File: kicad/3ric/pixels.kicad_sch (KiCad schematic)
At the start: 13 parts

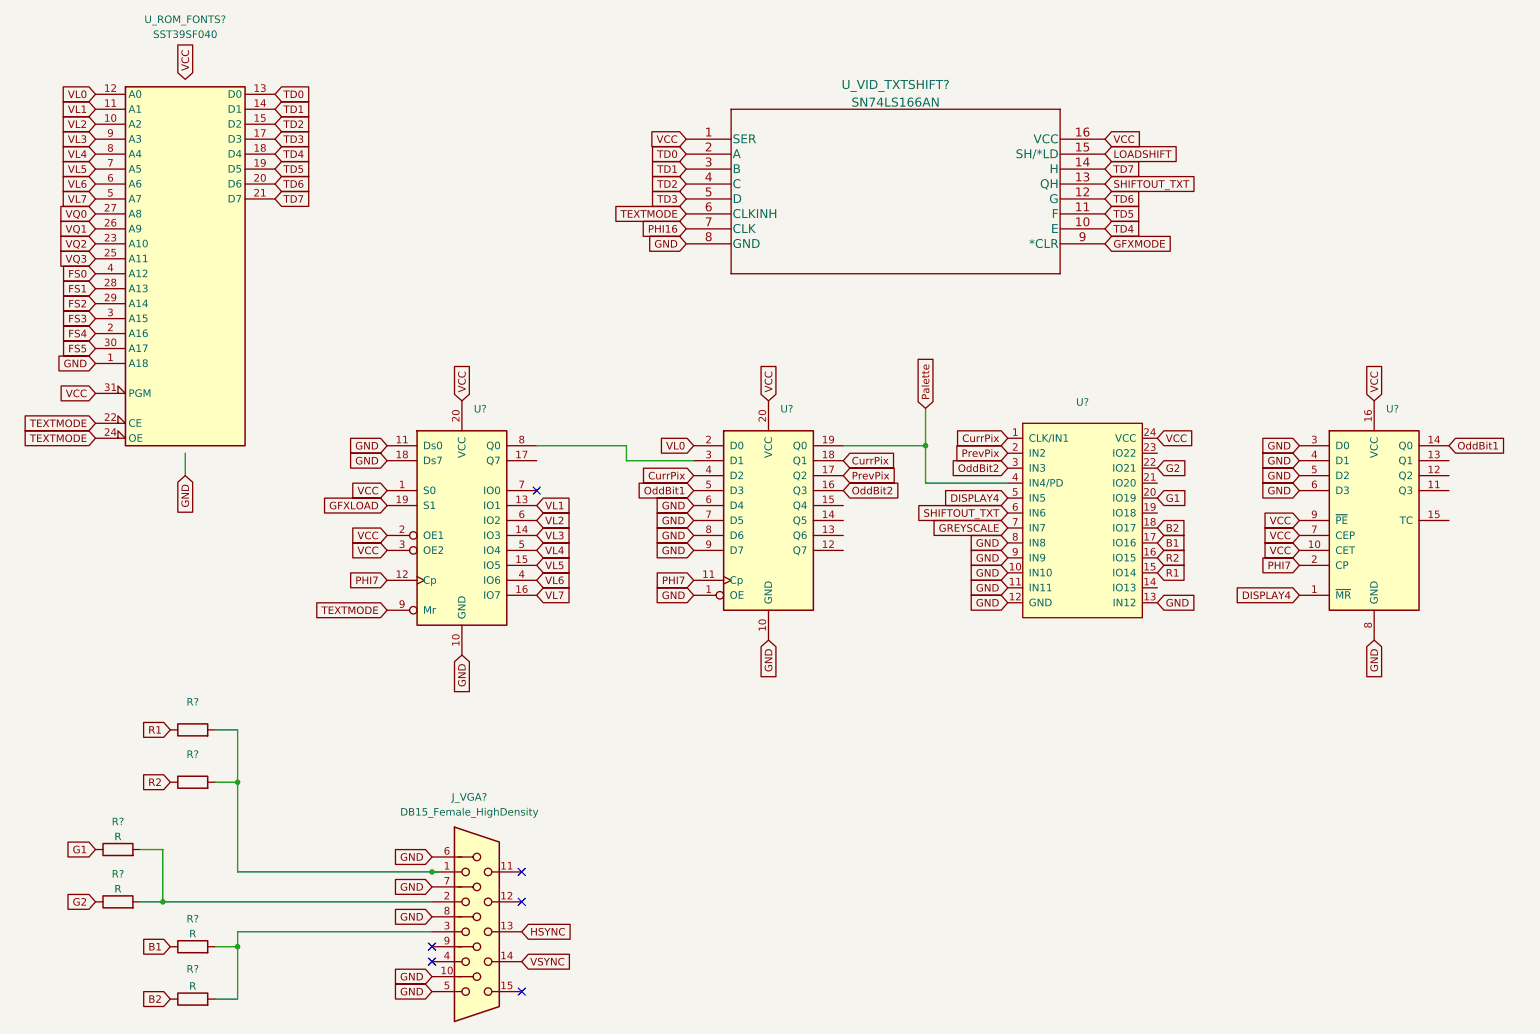
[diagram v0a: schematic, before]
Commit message: updates to logisim project and schematics
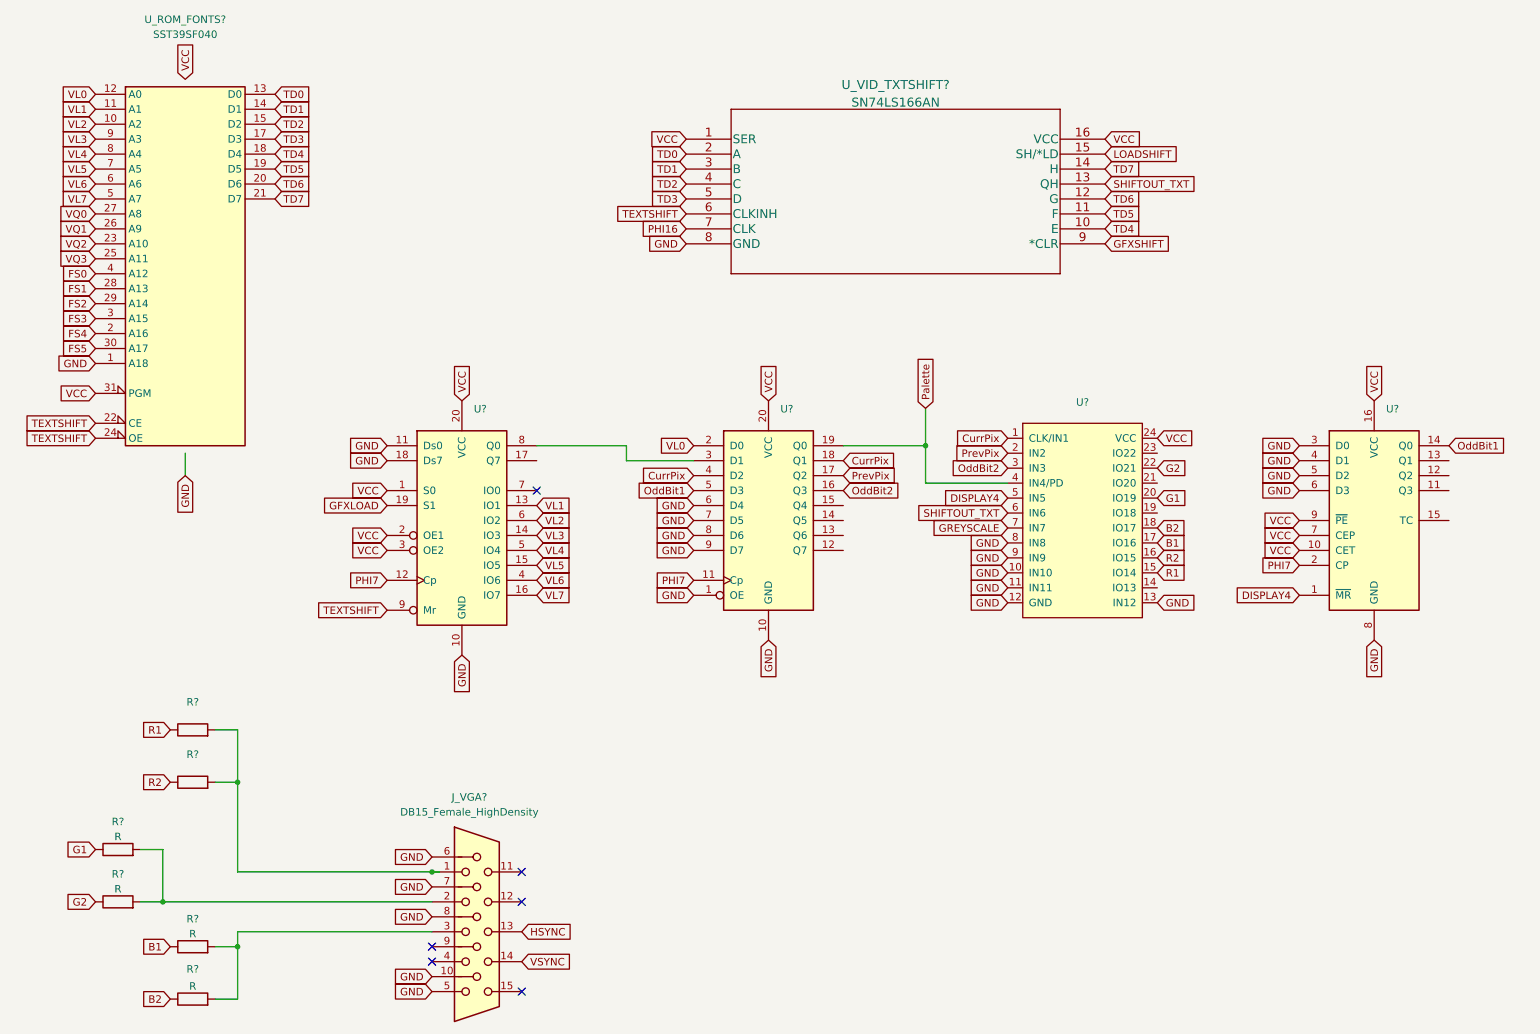
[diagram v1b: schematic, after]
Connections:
- net GFXMODE renamed GFXSHIFT
- net TEXTMODE renamed TEXTSHIFT
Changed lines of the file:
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@@
     )
   )
-  (global_label "TEXTMODE" (shape input) (at 82.55 119.38 180) (fields_autoplaced)
-    (effects (font (size 1.27 1.27)) (justify right))
-    (property "Intersheet References" "${INTERSHEET_REFS}" (id 0) (at 70.6421 119.4594 0)
+  (global_label "TEXTSHIFT" (shape input) (at 82.55 119.38 180) (fields_autoplaced)
+    (effects (font (size 1.27 1.27)) (justify right))
+    (property "Intersheet References" "${INTERSHEET_REFS}" (id 0) (at 70.6421 119.3006 0)
       (effects (font (size 1.27 1.27)) (justify right) hide)
     )
@@
     )
   )
-  (global_label "TEXTMODE" (shape input) (at 33.02 90.17 180) (fields_autoplaced)
-    (effects (font (size 1.27 1.27)) (justify right))
-    (property "Intersheet References" "${INTERSHEET_REFS}" (id 0) (at 21.1121 90.2494 0)
+  (global_label "TEXTSHIFT" (shape input) (at 33.02 90.17 180) (fields_autoplaced)
+    (effects (font (size 1.27 1.27)) (justify right))
+    (property "Intersheet References" "${INTERSHEET_REFS}" (id 0) (at 21.1121 90.0906 0)
       (effects (font (size 1.27 1.27)) (justify right) hide)
     )
@@
     )
   )
-  (global_label "TEXTMODE" (shape input) (at 33.02 87.63 180) (fields_autoplaced)
-    (effects (font (size 1.27 1.27)) (justify right))
-    (property "Intersheet References" "${INTERSHEET_REFS}" (id 0) (at 21.1121 87.7094 0)
+  (global_label "TEXTSHIFT" (shape input) (at 33.02 87.63 180) (fields_autoplaced)
+    (effects (font (size 1.27 1.27)) (justify right))
+    (property "Intersheet References" "${INTERSHEET_REFS}" (id 0) (at 21.1121 87.5506 0)
       (effects (font (size 1.27 1.27)) (justify right) hide)
     )
@@
     )
   )
-  (global_label "GFXMODE" (shape input) (at 204.47 57.15 0) (fields_autoplaced)
+  (global_label "GFXSHIFT" (shape input) (at 204.47 57.15 0) (fields_autoplaced)
     (effects (font (size 1.27 1.27)) (justify left))
     (property "Intersheet References" "${INTERSHEET_REFS}" (id 0) (at 215.6521 57.0706 0)
@@
     )
   )
-  (global_label "TEXTMODE" (shape input) (at 133.35 52.07 180) (fields_autoplaced)
+  (global_label "TEXTSHIFT" (shape input) (at 133.35 52.07 180) (fields_autoplaced)
     (effects (font (size 1.27 1.27)) (justify right))
     (property "Intersheet References" "${INTERSHEET_REFS}" (id 0) (at 121.4421 51.9906 0)

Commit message: push schematic updates
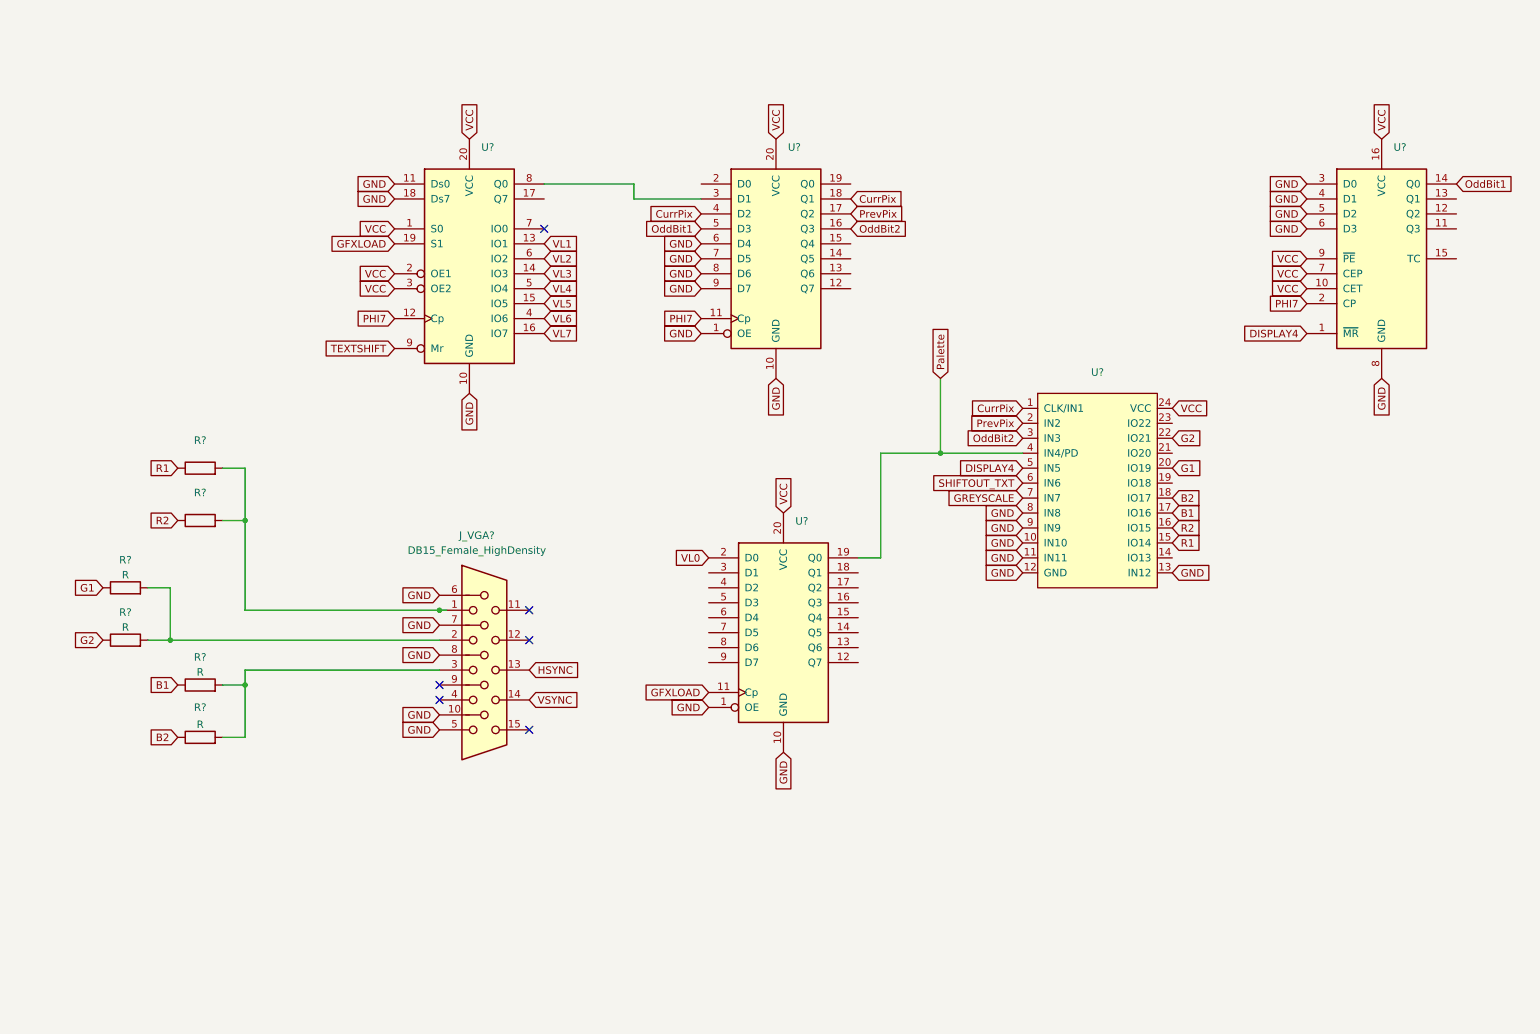
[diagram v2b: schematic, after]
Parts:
- removed U_ROM_FONTS?: SST39SF040, Package_DIP:DIP-32_W15.24mm_Socket, symbol Memory_Flash:SST39SF040
- removed U_VID_TXTSHIFT?: SN74LS166AN, Package_DIP:DIP-16_W7.62mm_Socket, symbol 74ls166:SN74LS166AN
- added U?: ~, symbol 74xx:74LS574
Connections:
- net GFXLOAD: now also U?.11 (Cp)
- net GND: now also U?.1 (OE), U?.10 (GND)
- net Palette: now also U?.19 (Q0); no longer U?.19 (Q0)
- net VCC: now also U?.20 (VCC)
- net VL0: now also U?.2 (D0); no longer U?.2 (D0)
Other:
- moved on the sheet: J_VGA?, R?, U?
